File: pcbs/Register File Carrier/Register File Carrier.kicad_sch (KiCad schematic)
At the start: 6 parts, among them J1001 Conn_02x20_Odd_Even, J1002 Conn_02x20_Odd_Even, U1001 74HC245, U1002 74HC245, U1003 74HC245, U1004 74HC245

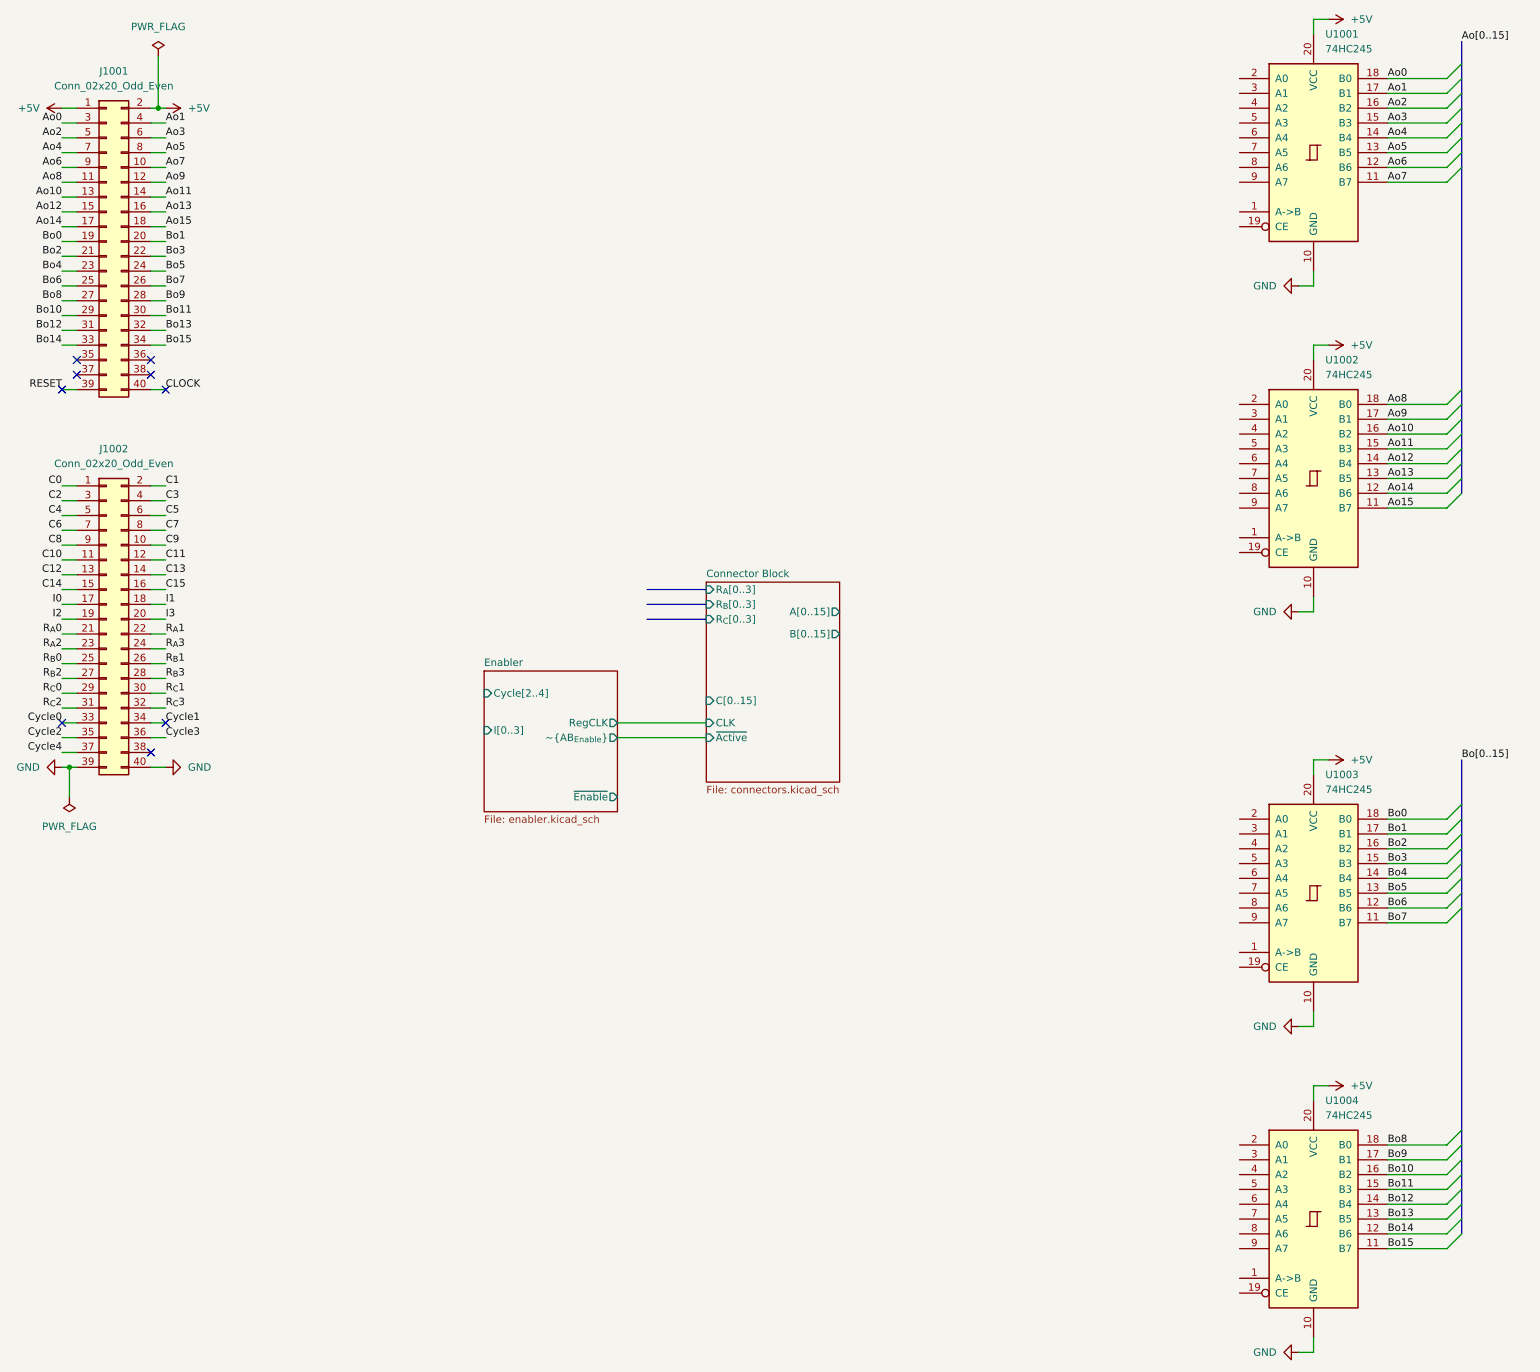
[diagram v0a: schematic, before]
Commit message: Starting to route
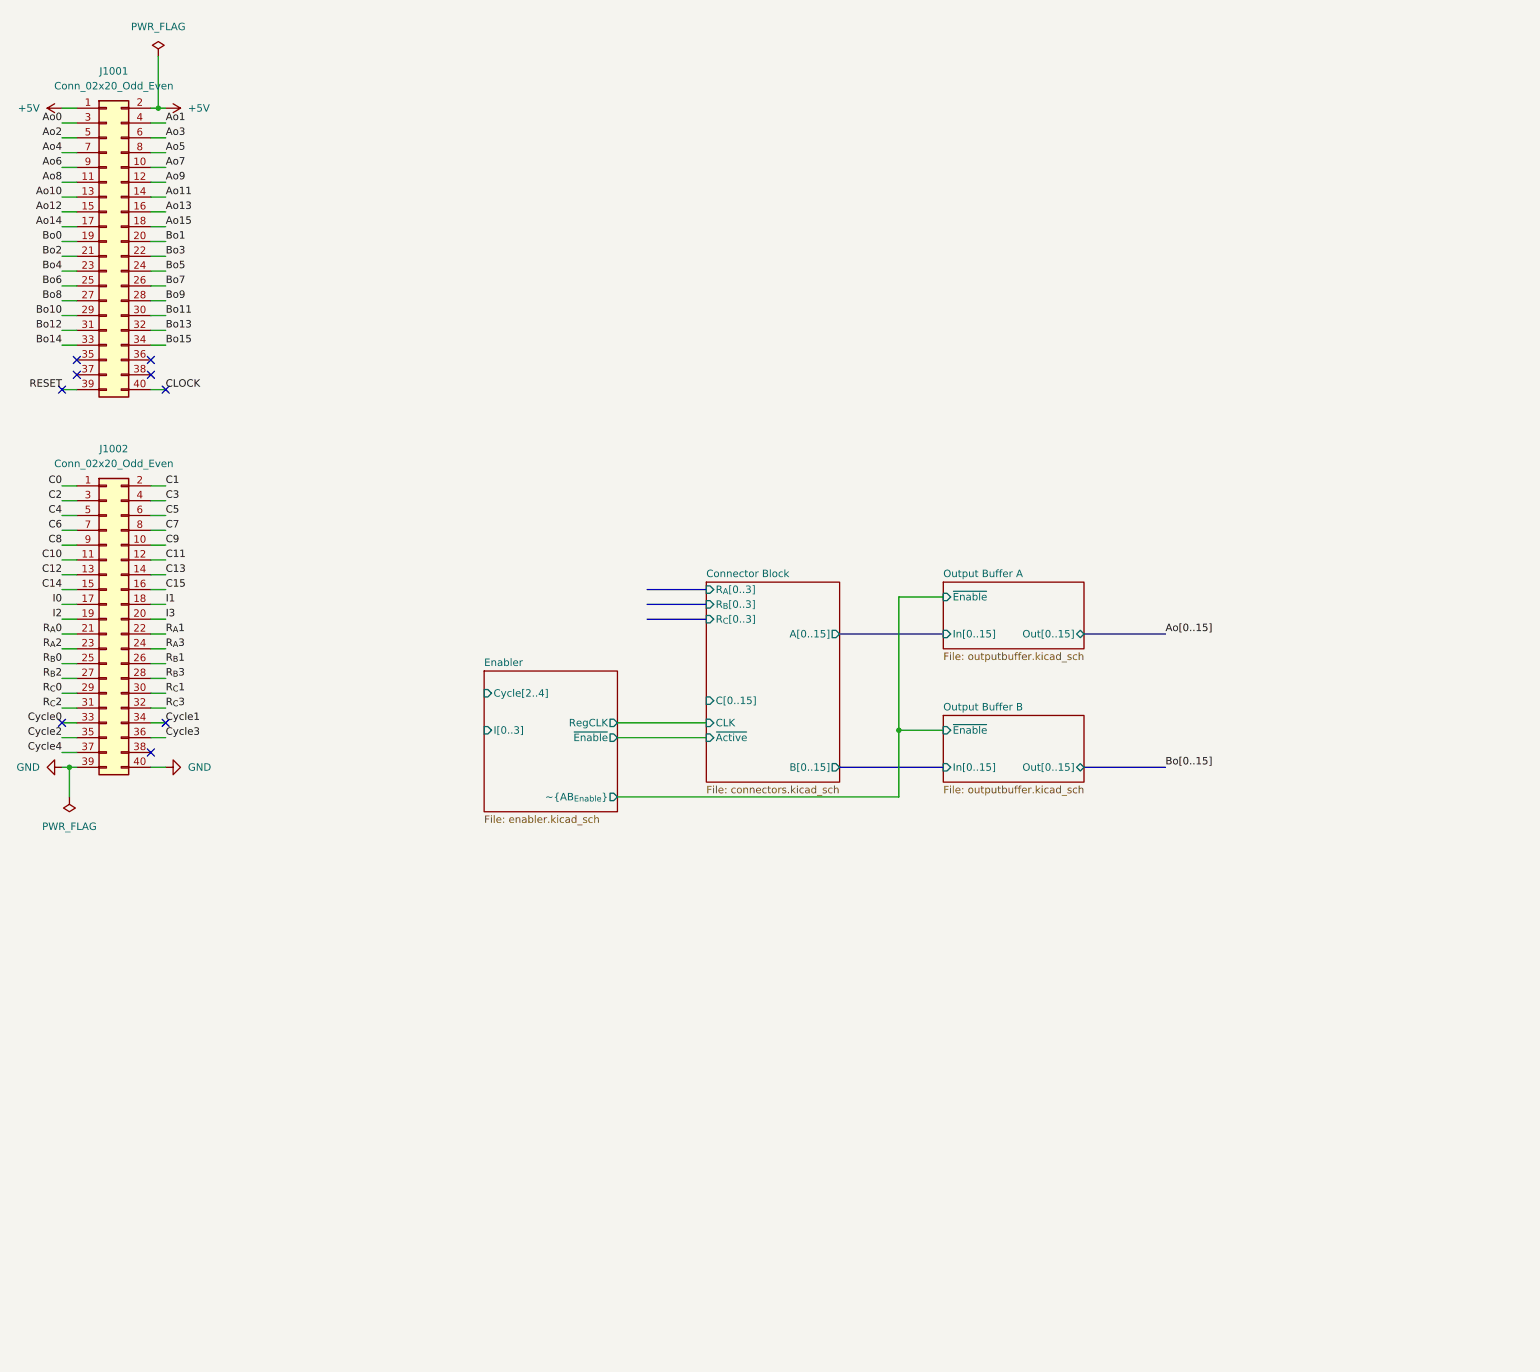
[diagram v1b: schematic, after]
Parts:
- removed U1001, U1002, U1003, U1004: 74HC245, Package_SO:SOIC-20W_7.5x12.8mm_P1.27mm, symbol 74xx:74HC245
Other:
- added sheet Output Buffer A (outputbuffer.kicad_sch)
- added sheet Output Buffer B (outputbuffer.kicad_sch)
